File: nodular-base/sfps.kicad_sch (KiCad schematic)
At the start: 24 parts, among them J1 Conn_02x10_Counter_Clockwise, J2 Conn_02x10_Counter_Clockwise, J3 Conn_02x10_Counter_Clockwise, J4 Conn_02x10_Counter_Clockwise, J5 Conn_02x10_Counter_Clockwise, J6 Conn_02x10_Counter_Clockwise, U10 MT9700, U11 MT9700, U12 MT9700, U13 MT9700, U8 MT9700, U9 MT9700

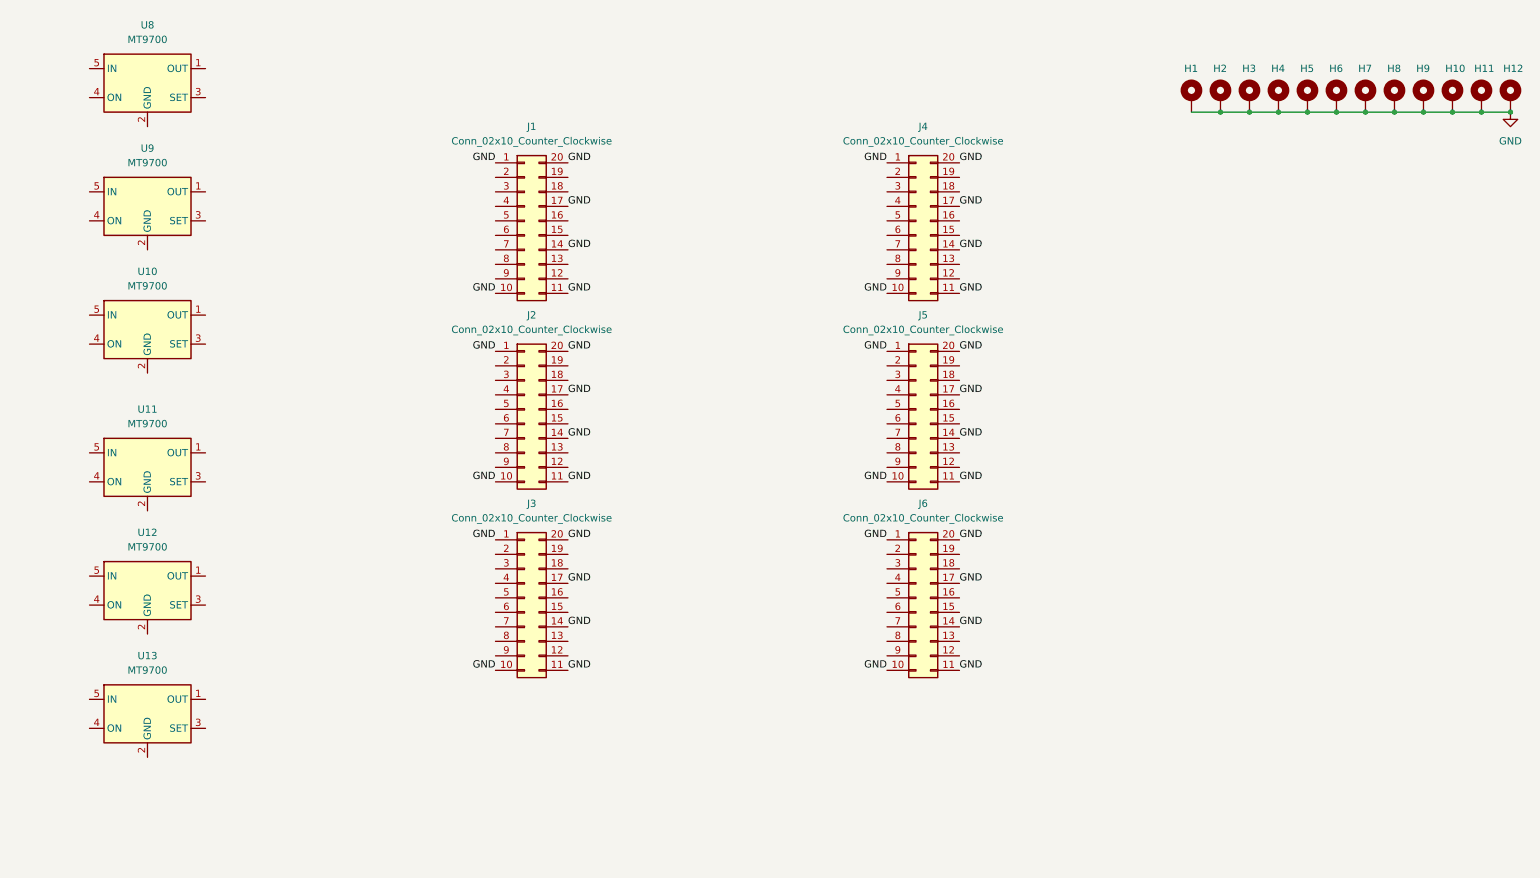
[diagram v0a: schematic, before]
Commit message: WIP layout for base
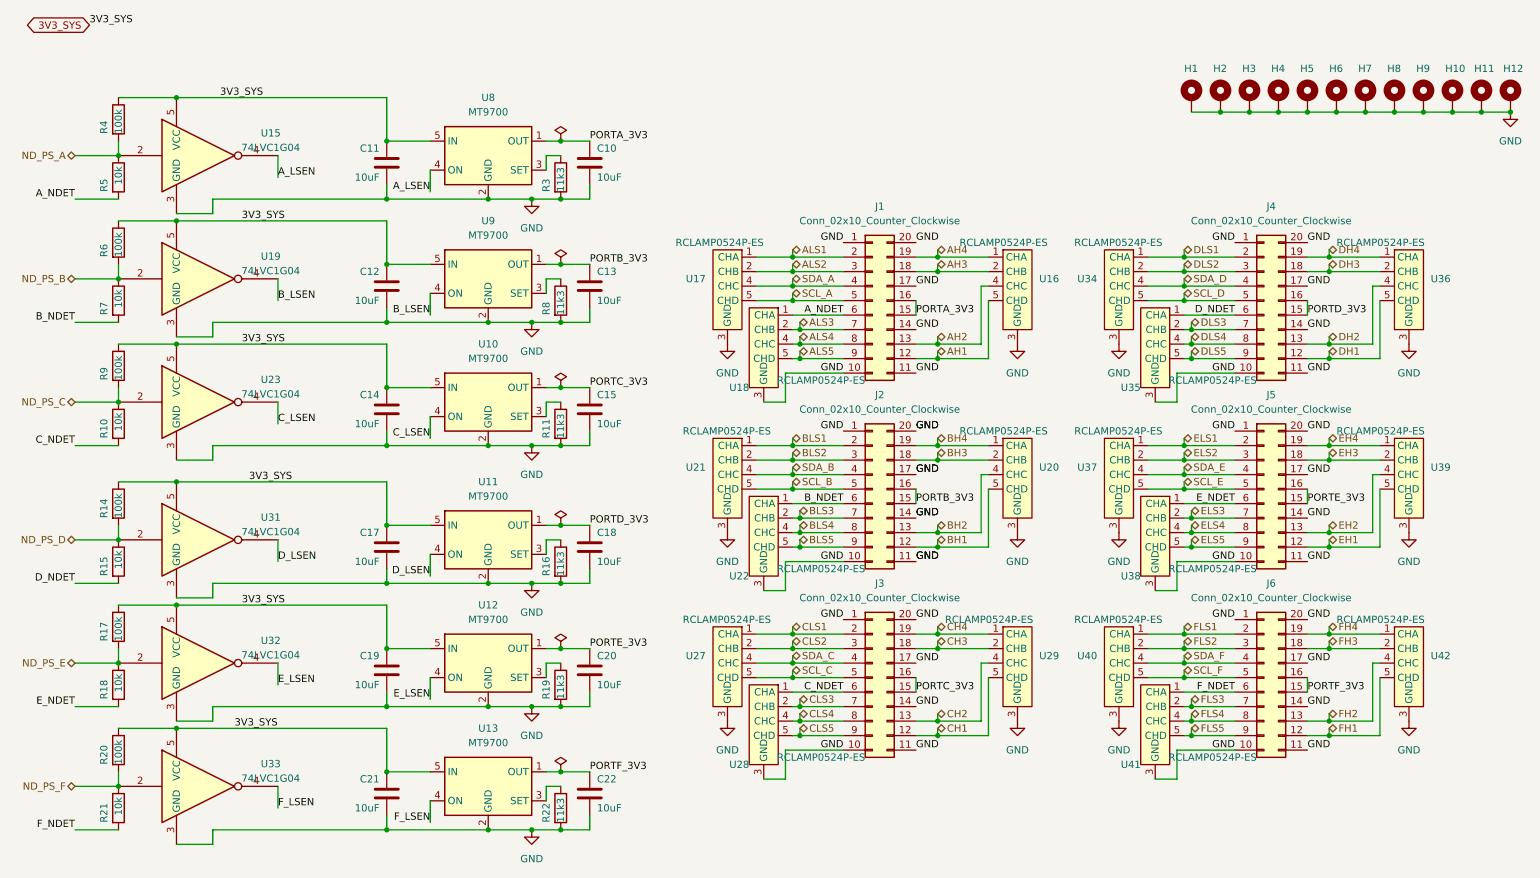
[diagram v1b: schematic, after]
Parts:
- added C10, C11, C12, C13, C14, C15, C17, C18, C19, C20, C21, C22: 10uF, Capacitor_SMD:C_1206_3216Metric, symbol Device:C
- added R10, R15, R18, R21, R5, R7: 10k, Resistor_SMD:R_0402_1005Metric, symbol Device:R
- added R11, R16, R19, R22, R3, R8: 11k3, Resistor_SMD:R_0402_1005Metric, symbol Device:R
- added R14, R17, R20, R4, R6, R9: 100k, Resistor_SMD:R_0402_1005Metric, symbol Device:R
- added U15, U19, U23, U31, U32, U33: 74LVC1G04, Package_TO_SOT_SMD:SOT-353_SC-70-5, symbol 74xGxx:74LVC1G04
- added U16, U17, U18, U20, U21, U22, U27, U28, U29, U34, U35, U36, U37, U38, U39, U40, U41, U42: RCLAMP0524P-ES, Package_DFN_QFN:Diodes_UDFN-10_1.0x2.5mm_P0.5mm, symbol nodular:RCLAMP0524P-ES
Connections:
- net GND: now also U10.2 (GND), U11.2 (GND), U12.2 (GND), U13.2 (GND), U8.2 (GND), U9.2 (GND), C10.2, C11.2, C12.2, C13.2, C14.2, C15.2, C17.2, C18.2, C19.2, C20.2, C21.2, C22.2, R11.2, R16.2, R19.2, R22.2, R3.2, R8.2, U15.3 (GND), U16.3 (GND), U16.8 (GND), U17.3 (GND), U17.8 (GND), U18.3 (GND), U18.8 (GND), U19.3 (GND), U20.3 (GND), U20.8 (GND), U21.3 (GND), U21.8 (GND), U22.3 (GND), U22.8 (GND), U23.3 (GND), U27.3 (GND), U27.8 (GND), U28.3 (GND), U28.8 (GND), U29.3 (GND), U29.8 (GND), U31.3 (GND), U32.3 (GND), U33.3 (GND), U34.3 (GND), U34.8 (GND), U35.3 (GND), U35.8 (GND), U36.3 (GND), U36.8 (GND), U37.3 (GND), U37.8 (GND), U38.3 (GND), U38.8 (GND), U39.3 (GND), U39.8 (GND), U40.3 (GND), U40.8 (GND), U41.3 (GND), U41.8 (GND), U42.3 (GND), U42.8 (GND)
- net BH1: now reaches J2.12 (Pin_12)
- net BH1: now also U20.5 (CHD), U20.6 (CHD)
- net BH2: now reaches J2.13 (Pin_13)
- net BH2: now also U20.4 (CHC), U20.7 (CHC)
- net PORTB_3V3: now reaches J2.15 (Pin_15)
- net PORTB_3V3: now also J2.16 (Pin_16), U9.1 (OUT), C13.1
- net BH3: now reaches J2.18 (Pin_18)
- net BH3: now also U20.2 (CHB), U20.9 (CHB)
- net BH4: now reaches J2.19 (Pin_19)
- net BH4: now also U20.1 (CHA), U20.10 (CHA)
- net BLS1: now reaches J2.2 (Pin_2)
- net BLS1: now also U21.1 (CHA), U21.10 (CHA)
- net BLS2: now reaches J2.3 (Pin_3)
- net BLS2: now also U21.2 (CHB), U21.9 (CHB)
- net SDA_B: now reaches J2.4 (Pin_4)
- net SDA_B: now also U21.4 (CHC), U21.7 (CHC)
- net SCL_B: now reaches J2.5 (Pin_5)
- net SCL_B: now also U21.5 (CHD), U21.6 (CHD)
- net B_NDET: now reaches J2.6 (Pin_6)
- net B_NDET: now also R7.2, U22.1 (CHA), U22.10 (CHA)
- net BLS3: now reaches J2.7 (Pin_7)
- net BLS3: now also U22.2 (CHB), U22.9 (CHB)
- net BLS4: now reaches J2.8 (Pin_8)
- net BLS4: now also U22.4 (CHC), U22.7 (CHC)
- net BLS5: now reaches J2.9 (Pin_9)
- net BLS5: now also U22.5 (CHD), U22.6 (CHD)
- net EH1: now reaches J5.12 (Pin_12)
- net EH1: now also U39.5 (CHD), U39.6 (CHD)
- net EH2: now reaches J5.13 (Pin_13)
- net EH2: now also U39.4 (CHC), U39.7 (CHC)
- net PORTE_3V3: now reaches J5.15 (Pin_15)
- net PORTE_3V3: now also J5.16 (Pin_16), U12.1 (OUT), C20.1
- net EH3: now reaches J5.18 (Pin_18)
- net EH3: now also U39.2 (CHB), U39.9 (CHB)
- net EH4: now reaches J5.19 (Pin_19)
- net EH4: now also U39.1 (CHA), U39.10 (CHA)
- net ELS1: now reaches J5.2 (Pin_2)
- net ELS1: now also U37.1 (CHA), U37.10 (CHA)
- net ELS2: now reaches J5.3 (Pin_3)
- net ELS2: now also U37.2 (CHB), U37.9 (CHB)
- net SDA_E: now reaches J5.4 (Pin_4)
- net SDA_E: now also U37.4 (CHC), U37.7 (CHC)
- net SCL_E: now reaches J5.5 (Pin_5)
- net SCL_E: now also U37.5 (CHD), U37.6 (CHD)
- net E_NDET: now reaches J5.6 (Pin_6)
- net E_NDET: now also R18.2, U38.1 (CHA), U38.10 (CHA)
- net ELS3: now reaches J5.7 (Pin_7)
- net ELS3: now also U38.2 (CHB), U38.9 (CHB)
- net ELS4: now reaches J5.8 (Pin_8)
- net ELS4: now also U38.4 (CHC), U38.7 (CHC)
- net ELS5: now reaches J5.9 (Pin_9)
- net ELS5: now also U38.5 (CHD), U38.6 (CHD)
- net AH1: now reaches J1.12 (Pin_12)
- net AH1: now also U16.5 (CHD), U16.6 (CHD)
- net AH2: now reaches J1.13 (Pin_13)
- net AH2: now also U16.4 (CHC), U16.7 (CHC)
- net PORTA_3V3: now reaches J1.15 (Pin_15)
- net PORTA_3V3: now also J1.16 (Pin_16), U8.1 (OUT), C10.1
- net AH3: now reaches J1.18 (Pin_18)
- net AH3: now also U16.2 (CHB), U16.9 (CHB)
- net AH4: now reaches J1.19 (Pin_19)
- net AH4: now also U16.1 (CHA), U16.10 (CHA)
- net ALS1: now reaches J1.2 (Pin_2)
- net ALS1: now also U17.1 (CHA), U17.10 (CHA)
- net ALS2: now reaches J1.3 (Pin_3)
- net ALS2: now also U17.2 (CHB), U17.9 (CHB)
- net SDA_A: now reaches J1.4 (Pin_4)
- net SDA_A: now also U17.4 (CHC), U17.7 (CHC)
- net SCL_A: now reaches J1.5 (Pin_5)
- net SCL_A: now also U17.5 (CHD), U17.6 (CHD)
- net A_NDET: now reaches J1.6 (Pin_6)
- net A_NDET: now also R5.2, U18.1 (CHA), U18.10 (CHA)
- net ALS3: now reaches J1.7 (Pin_7)
- net ALS3: now also U18.2 (CHB), U18.9 (CHB)
- net ALS4: now reaches J1.8 (Pin_8)
- net ALS4: now also U18.4 (CHC), U18.7 (CHC)
- net ALS5: now reaches J1.9 (Pin_9)
- net ALS5: now also U18.5 (CHD), U18.6 (CHD)
- net DH1: now reaches J4.12 (Pin_12)
- net DH1: now also U36.5 (CHD), U36.6 (CHD)
- net DH2: now reaches J4.13 (Pin_13)
- net DH2: now also U36.4 (CHC), U36.7 (CHC)
- net PORTD_3V3: now reaches J4.15 (Pin_15)
- net PORTD_3V3: now also J4.16 (Pin_16), U11.1 (OUT), C18.1
- net DH3: now reaches J4.18 (Pin_18)
- net DH3: now also U36.2 (CHB), U36.9 (CHB)
- net DH4: now reaches J4.19 (Pin_19)
- net DH4: now also U36.1 (CHA), U36.10 (CHA)
- net DLS1: now reaches J4.2 (Pin_2)
- net DLS1: now also U34.1 (CHA), U34.10 (CHA)
- net DLS2: now reaches J4.3 (Pin_3)
- net DLS2: now also U34.2 (CHB), U34.9 (CHB)
- net SDA_D: now reaches J4.4 (Pin_4)
- net SDA_D: now also U34.4 (CHC), U34.7 (CHC)
- net SCL_D: now reaches J4.5 (Pin_5)
- net SCL_D: now also U34.5 (CHD), U34.6 (CHD)
- net D_NDET: now reaches J4.6 (Pin_6)
- net D_NDET: now also R15.2, U35.1 (CHA), U35.10 (CHA)
- net DLS3: now reaches J4.7 (Pin_7)
- net DLS3: now also U35.2 (CHB), U35.9 (CHB)
- net DLS4: now reaches J4.8 (Pin_8)
- net DLS4: now also U35.4 (CHC), U35.7 (CHC)
- net DLS5: now reaches J4.9 (Pin_9)
- net DLS5: now also U35.5 (CHD), U35.6 (CHD)
- net at U11.3 (SET): now also R16.1
- net D_LSEN: now reaches U11.4 (ON)
- net D_LSEN: now also U31.4
- net 3V3_SYS: now reaches U11.5 (IN)
- net 3V3_SYS: now also U10.5 (IN), U12.5 (IN), U13.5 (IN), U8.5 (IN), U9.5 (IN), C11.1, C12.1, C14.1, C17.1, C19.1, C21.1, R14.1, R17.1, R20.1, R4.1, R6.1, R9.1, U15.5 (VCC), U19.5 (VCC), U23.5 (VCC), U31.5 (VCC), U32.5 (VCC), U33.5 (VCC)
- net CH1: now reaches J3.12 (Pin_12)
- net CH1: now also U29.5 (CHD), U29.6 (CHD)
- net CH2: now reaches J3.13 (Pin_13)
- net CH2: now also U29.4 (CHC), U29.7 (CHC)
- net PORTC_3V3: now reaches J3.15 (Pin_15)
- net PORTC_3V3: now also J3.16 (Pin_16), U10.1 (OUT), C15.1
- net CH3: now reaches J3.18 (Pin_18)
- net CH3: now also U29.2 (CHB), U29.9 (CHB)
- net CH4: now reaches J3.19 (Pin_19)
- net CH4: now also U29.1 (CHA), U29.10 (CHA)
- net CLS1: now reaches J3.2 (Pin_2)
- net CLS1: now also U27.1 (CHA), U27.10 (CHA)
- net CLS2: now reaches J3.3 (Pin_3)
- net CLS2: now also U27.2 (CHB), U27.9 (CHB)
- net SDA_C: now reaches J3.4 (Pin_4)
- net SDA_C: now also U27.4 (CHC), U27.7 (CHC)
- net SCL_C: now reaches J3.5 (Pin_5)
- net SCL_C: now also U27.5 (CHD), U27.6 (CHD)
- net C_NDET: now reaches J3.6 (Pin_6)
- net C_NDET: now also R10.2, U28.1 (CHA), U28.10 (CHA)
- net CLS3: now reaches J3.7 (Pin_7)
- net CLS3: now also U28.2 (CHB), U28.9 (CHB)
- net CLS4: now reaches J3.8 (Pin_8)
- net CLS4: now also U28.4 (CHC), U28.7 (CHC)
- net CLS5: now reaches J3.9 (Pin_9)
- net CLS5: now also U28.5 (CHD), U28.6 (CHD)
- net at U9.3 (SET): now also R8.1
- net B_LSEN: now reaches U9.4 (ON)
- net B_LSEN: now also U19.4
- net at U12.3 (SET): now also R19.1
- net E_LSEN: now reaches U12.4 (ON)
- net E_LSEN: now also U32.4
- net at U8.3 (SET): now also R3.1
- net A_LSEN: now reaches U8.4 (ON)
- net A_LSEN: now also U15.4
- net at U10.3 (SET): now also R11.1
- net C_LSEN: now reaches U10.4 (ON)
- net C_LSEN: now also U23.4
- net FH1: now reaches J6.12 (Pin_12)
- net FH1: now also U42.5 (CHD), U42.6 (CHD)
- net FH2: now reaches J6.13 (Pin_13)
- net FH2: now also U42.4 (CHC), U42.7 (CHC)
- net PORTF_3V3: now reaches J6.15 (Pin_15)
- net PORTF_3V3: now also J6.16 (Pin_16), U13.1 (OUT), C22.1
- net FH3: now reaches J6.18 (Pin_18)
- net FH3: now also U42.2 (CHB), U42.9 (CHB)
- net FH4: now reaches J6.19 (Pin_19)
- net FH4: now also U42.1 (CHA), U42.10 (CHA)
- net FLS1: now reaches J6.2 (Pin_2)
- net FLS1: now also U40.1 (CHA), U40.10 (CHA)
- net FLS2: now reaches J6.3 (Pin_3)
- net FLS2: now also U40.2 (CHB), U40.9 (CHB)
- net SDA_F: now reaches J6.4 (Pin_4)
- net SDA_F: now also U40.4 (CHC), U40.7 (CHC)
- net SCL_F: now reaches J6.5 (Pin_5)
- net SCL_F: now also U40.5 (CHD), U40.6 (CHD)
- net F_NDET: now reaches J6.6 (Pin_6)
- net F_NDET: now also R21.2, U41.1 (CHA), U41.10 (CHA)
- net FLS3: now reaches J6.7 (Pin_7)
- net FLS3: now also U41.2 (CHB), U41.9 (CHB)
- net FLS4: now reaches J6.8 (Pin_8)
- net FLS4: now also U41.4 (CHC), U41.7 (CHC)
- net FLS5: now reaches J6.9 (Pin_9)
- net FLS5: now also U41.5 (CHD), U41.6 (CHD)
- net at U13.3 (SET): now also R22.1
- net F_LSEN: now reaches U13.4 (ON)
- net F_LSEN: now also U33.4
- new net ND_PS_A: R4.2, R5.1, U15.2
- new net ND_PS_B: R6.2, R7.1, U19.2
- new net ND_PS_C: R10.1, R9.2, U23.2
- new net ND_PS_D: R14.2, R15.1, U31.2
- new net ND_PS_E: R17.2, R18.1, U32.2
- new net ND_PS_F: R20.2, R21.1, U33.2
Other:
- moved on the sheet: J1, J2, J3, J4, J5, J6, U10, U11, U12, U13, U8, U9
